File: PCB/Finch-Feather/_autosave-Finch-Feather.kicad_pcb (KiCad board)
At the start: 4 copper layers, 61 x 22.9 mm, 36 parts, among them M1 STM32WB5MMGH6TR, Q1 DMP3125L-7, SW1 B3U-1000P, T1 20021121-00010C4LF, T2 TSW-112-07-G-S, T3 DX07S016JA1R1500, T4 TSW-116-07-L-S, T5 S2B-PH-SM4-TB(LF)(SN), U1 USBLC6-2P6, U2 TLV75533PDBVR, U3 MCP73831T-2ACI_OT

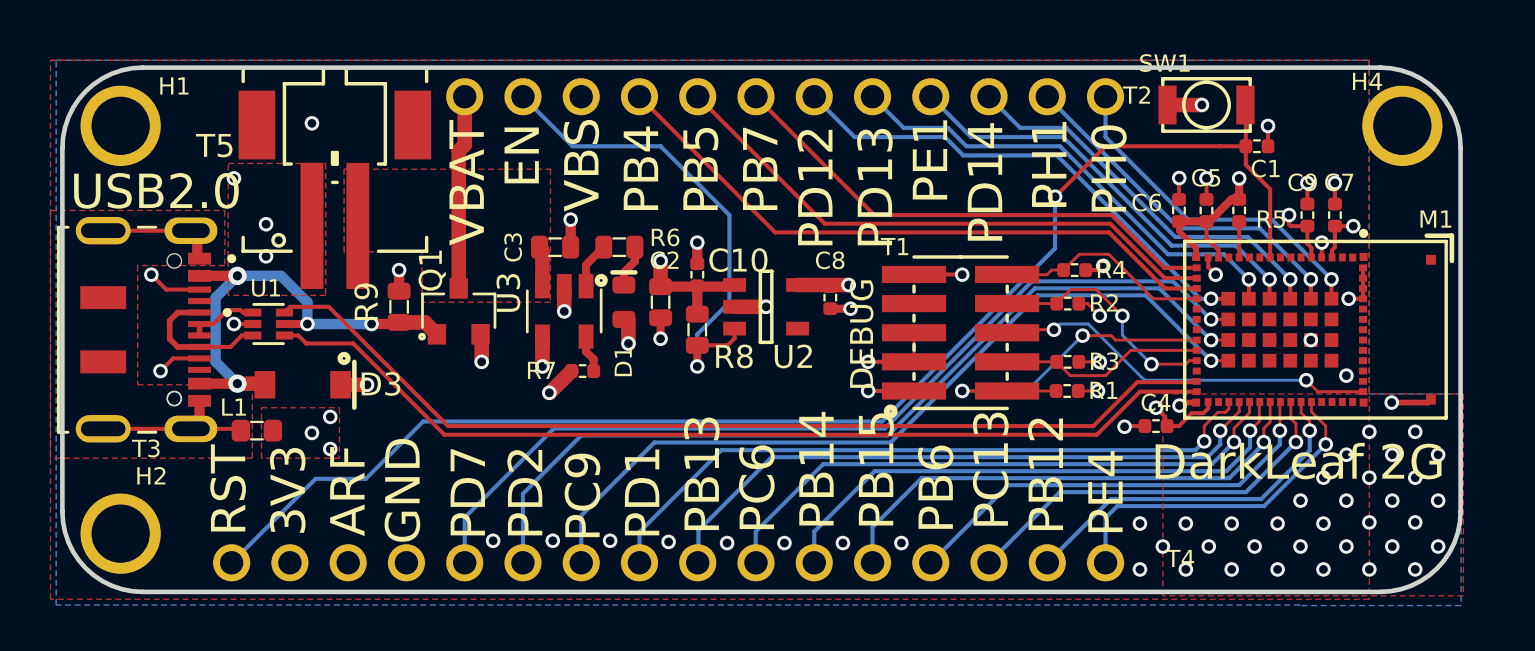
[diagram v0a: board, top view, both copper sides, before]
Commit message: PCB changes
Adjusted pours, next need to perfrom DRC, syncing for work
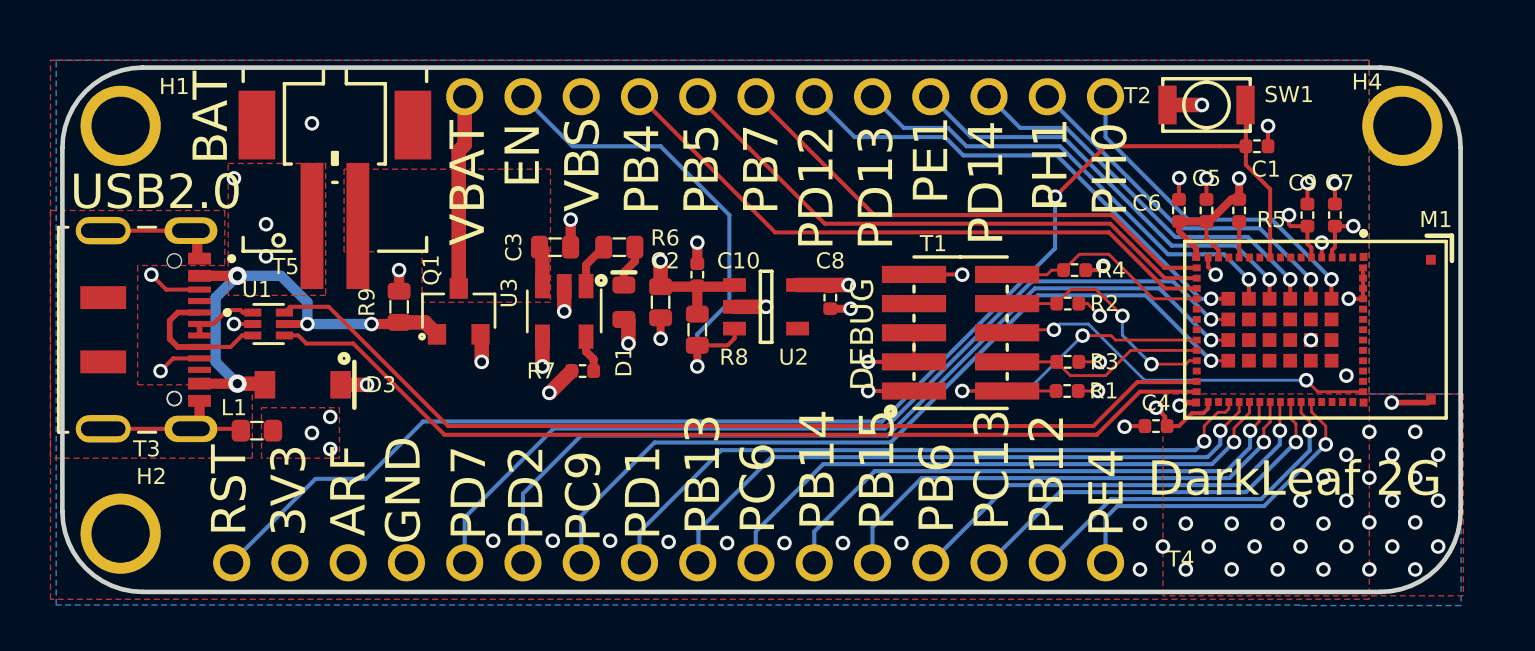
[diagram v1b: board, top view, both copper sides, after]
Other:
- board text added: "BAT"
